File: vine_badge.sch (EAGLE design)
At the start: 44 parts

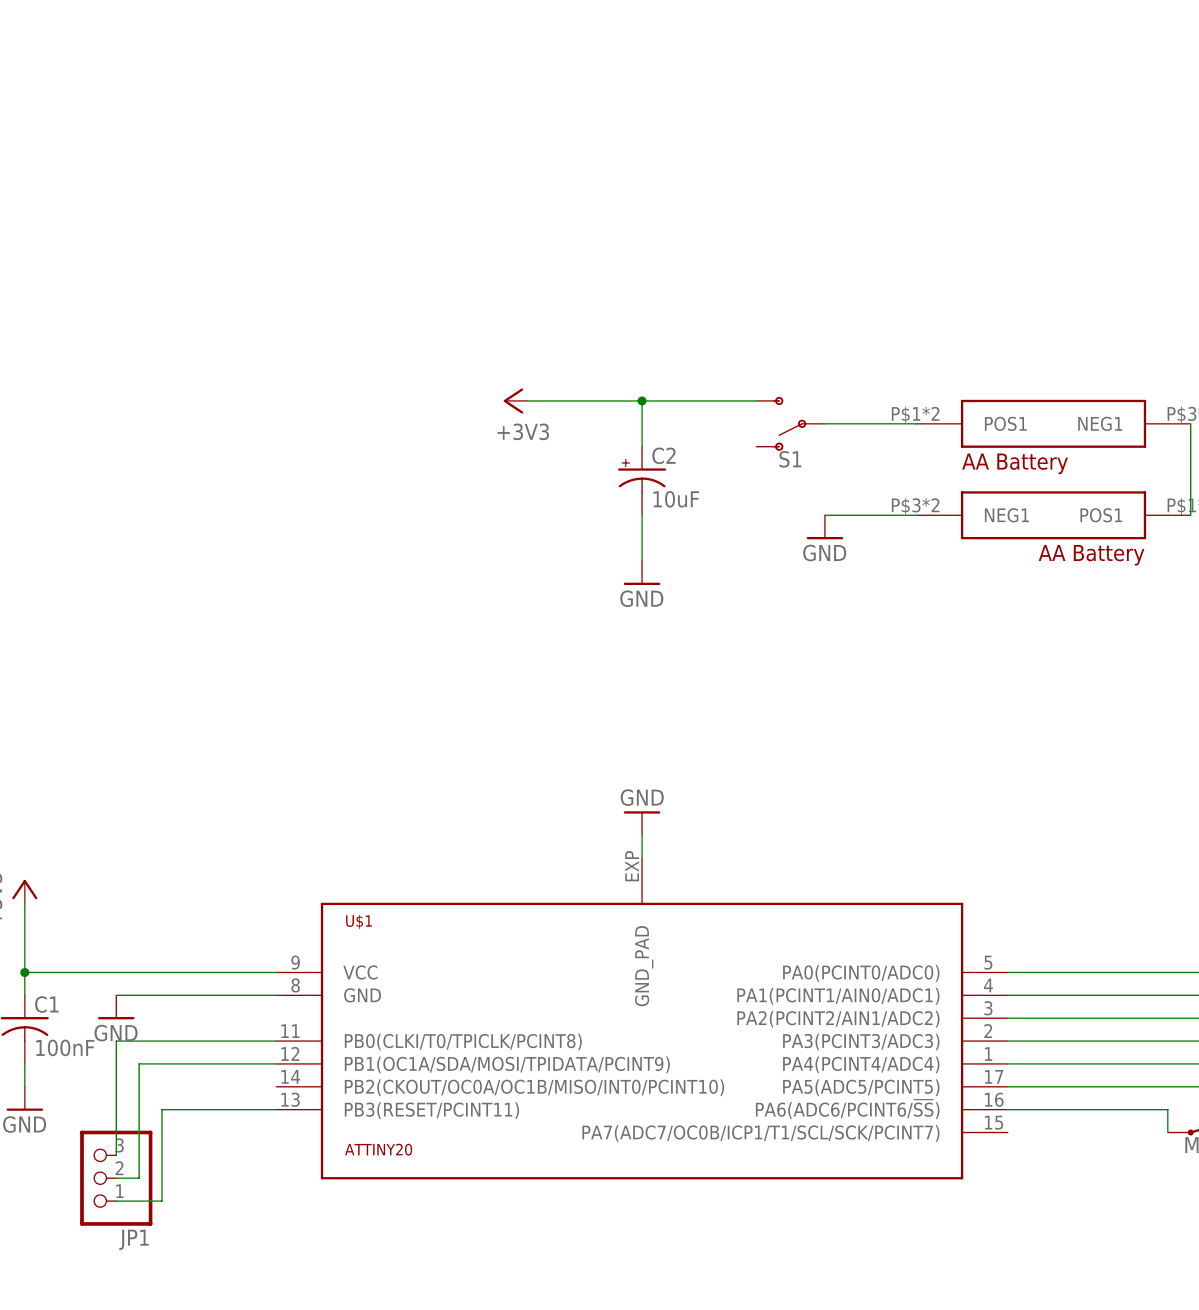
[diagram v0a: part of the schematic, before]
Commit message: final checking phase
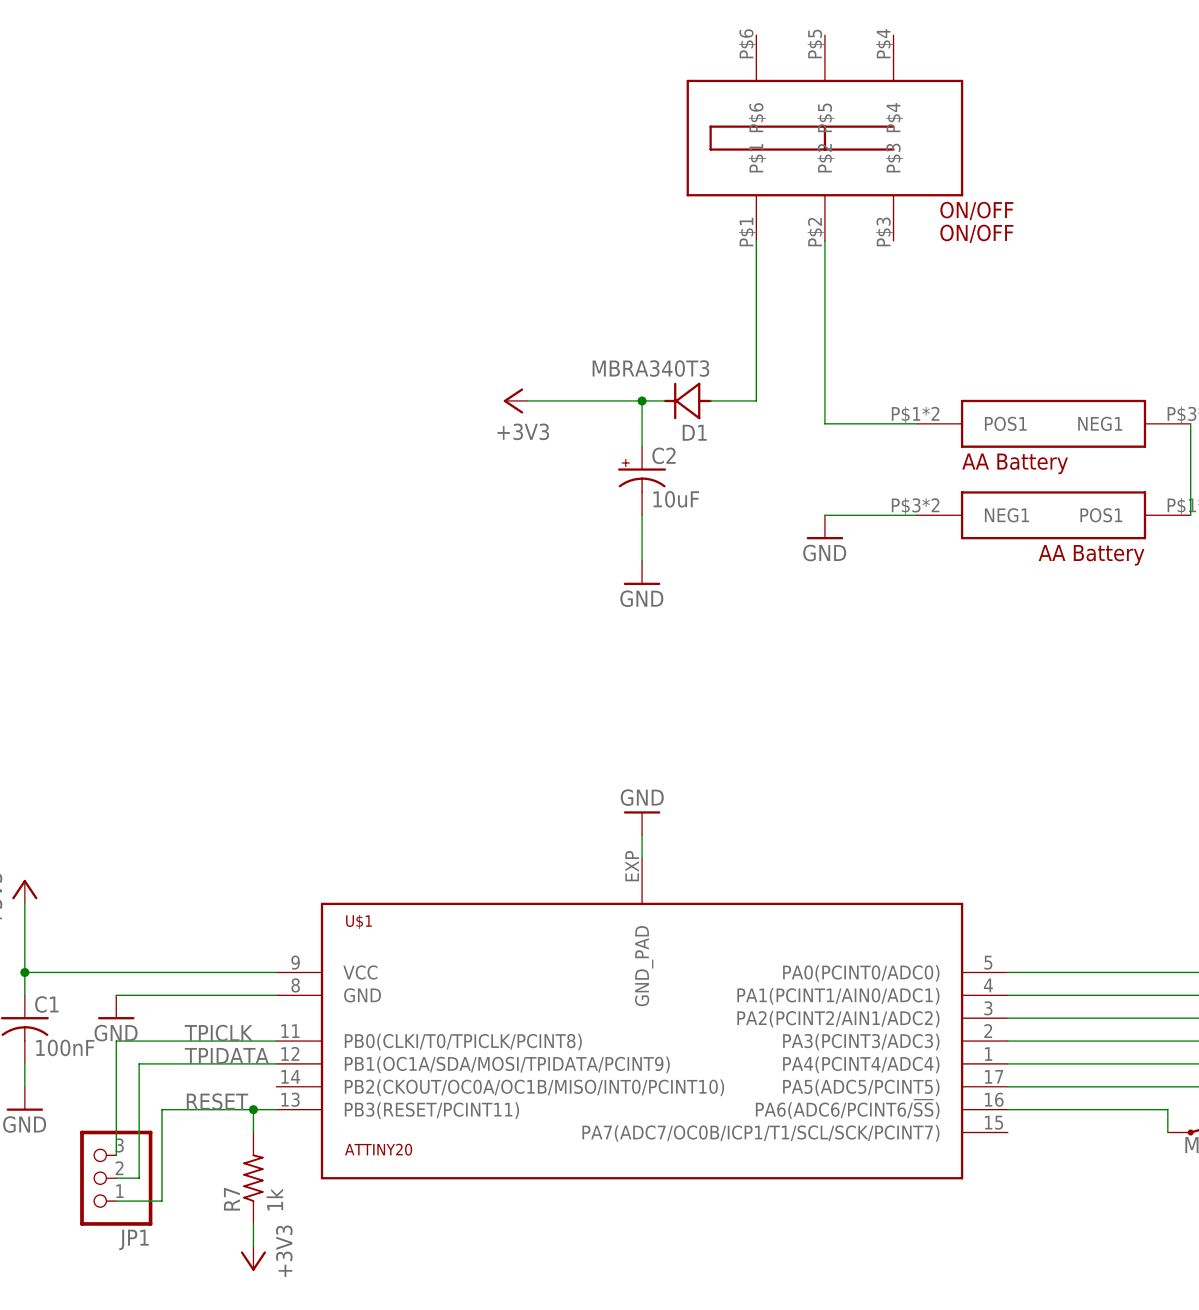
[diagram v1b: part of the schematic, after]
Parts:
- removed S1: (no value), SparkFun-Switches:SWITCH-SPDT-SMD-AYZ0202
- added D1: MBRA340T3, diode:MBRA340T3
- added ON/OFF: ON/OFF, VineBadge:SMT_DPDT
- added R7: 1k, resistor:R-US_R0603
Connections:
- net N$10 renamed TPIDATA
- net N$8 renamed TPICLK
- removed net N$12: JP1.1, U$1G$2.PB3(RESET/PCINT11)
- new net N$20: D1.A, ON/OFF.P$1
- new net RESET: JP1.1, R7.2, U$1G$2.PB3(RESET/PCINT11)
- net +3V3: now also D1.C, R7.1; no longer S1.S
- net N$19: now also ON/OFF.P$2; no longer S1.P
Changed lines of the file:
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@@
 <part name="C1" library="resistor" library_urn="urn:adsk.eagle:library:348" deviceset="C-US" device="C0603" package3d_urn="urn:adsk.eagle:package:23616/2" value="100nF"/>
 <part name="GND3" library="supply1" library_urn="urn:adsk.eagle:library:371" deviceset="GND" device=""/>
-<part name="S1" library="SparkFun-Switches" library_urn="urn:adsk.eagle:library:535" deviceset="SWITCH-SPDT" device="-SMD-AYZ0202" package3d_urn="urn:adsk.eagle:package:40160/1"/>
 <part name="+3V2" library="supply1" library_urn="urn:adsk.eagle:library:371" deviceset="+3V3" device=""/>
 <part name="GND4" library="supply1" library_urn="urn:adsk.eagle:library:371" deviceset="GND" device=""/>
@@
 <part name="S2" library="SparkFun-Switches" library_urn="urn:adsk.eagle:library:535" deviceset="MOMENTARY-SWITCH-SPST" device="-SMD-6.0X3.5MM" package3d_urn="urn:adsk.eagle:package:40165/1" value="MODE"/>
 <part name="JP1" library="pinhead" library_urn="urn:adsk.eagle:library:325" deviceset="PINHD-1X3" device="" package3d_urn="urn:adsk.eagle:package:22458/2"/>
+<part name="D1" library="diode" library_urn="urn:adsk.eagle:library:210" deviceset="MBRA340T3" device="" package3d_urn="urn:adsk.eagle:package:43460/3"/>
+<part name="R7" library="resistor" library_urn="urn:adsk.eagle:library:348" deviceset="R-US_" device="R0603" package3d_urn="urn:adsk.eagle:package:23555/2" value="1k"/>
+<part name="+3V3" library="supply1" library_urn="urn:adsk.eagle:library:371" deviceset="+3V3" device=""/>
+<part name="ON/OFF" library="VineBadge" deviceset="SMT_DPDT" device="" value="ON/OFF"/>
 </parts>
 <sheets>
@@
 <attribute name="VALUE" x="17.78" y="25.4" size="1.778" layer="96"/>
 </instance>
-<instance part="S1" gate="1" x="106.68" y="104.14" smashed="yes" rot="R180">
-<attribute name="NAME" x="105.41" y="101.092" size="1.778" layer="95" font="vector" rot="R180" align="bottom-center"/>
-<attribute name="VALUE" x="105.664" y="107.442" size="1.778" layer="96" font="vector" rot="R180" align="top-center"/>
-</instance>
 <instance part="+3V2" gate="G$1" x="73.66" y="106.68" smashed="yes" rot="R90">
 <attribute name="VALUE" x="78.74" y="104.14" size="1.778" layer="96" rot="R180"/>
@@
 <attribute name="NAME" x="34.29" y="14.605" size="1.778" layer="95" rot="R180"/>
 <attribute name="VALUE" x="34.29" y="27.94" size="1.778" layer="96" rot="R180"/>
+</instance>
+<instance part="D1" gate="G$1" x="93.98" y="106.68" smashed="yes" rot="R180">
+<attribute name="NAME" x="96.2914" y="104.0384" size="1.778" layer="95" rot="R180"/>
+<attribute name="VALUE" x="96.5454" y="111.1758" size="1.778" layer="96" rot="R180"/>
+</instance>
+<instance part="R7" gate="G$1" x="45.72" y="20.32" smashed="yes" rot="R90">
+<attribute name="NAME" x="44.2214" y="16.51" size="1.778" layer="95" rot="R90"/>
+<attribute name="VALUE" x="49.022" y="16.51" size="1.778" layer="96" rot="R90"/>
+</instance>
+<instance part="+3V3" gate="G$1" x="45.72" y="10.16" smashed="yes" rot="R180">
+<attribute name="VALUE" x="48.26" y="15.24" size="1.778" layer="96" rot="R270"/>
+</instance>
+<instance part="ON/OFF" gate="G$1" x="109.22" y="129.54" smashed="yes">
+<attribute name="NAME" x="121.92" y="127" size="1.778" layer="94"/>
+<attribute name="VALUE" x="121.92" y="124.46" size="1.778" layer="94"/>
 </instance>
 </instances>
@@
 </segment>
 <segment>
-<pinref part="S1" gate="1" pin="S"/>
 <pinref part="+3V2" gate="G$1" pin="+3V3"/>
-<wire x1="101.6" y1="106.68" x2="88.9" y2="106.68" width="0.1524" layer="91"/>
 <pinref part="C2" gate="G$1" pin="+"/>
 <wire x1="88.9" y1="106.68" x2="76.2" y2="106.68" width="0.1524" layer="91"/>
 <wire x1="88.9" y1="101.6" x2="88.9" y2="106.68" width="0.1524" layer="91"/>
+<pinref part="D1" gate="G$1" pin="C"/>
+<wire x1="91.44" y1="106.68" x2="88.9" y2="106.68" width="0.1524" layer="91"/>
 <junction x="88.9" y="106.68"/>
+</segment>
+<segment>
+<pinref part="R7" gate="G$1" pin="1"/>
+<pinref part="+3V3" gate="G$1" pin="+3V3"/>
+<wire x1="45.72" y1="15.24" x2="45.72" y2="12.7" width="0.1524" layer="91"/>
 </segment>
 </net>
@@
 </segment>
 </net>
-<net name="N$8" class="0">
+<net name="TPICLK" class="0">
 <segment>
 <pinref part="U$1" gate="G$2" pin="PB0(CLKI/T0/TPICLK/PCINT8)"/>
@@
 <pinref part="JP1" gate="A" pin="3"/>
 <wire x1="30.48" y1="35.56" x2="30.48" y2="22.86" width="0.1524" layer="91"/>
-</segment>
-</net>
-<net name="N$10" class="0">
+<label x="38.1" y="35.56" size="1.778" layer="95"/>
+</segment>
+</net>
+<net name="TPIDATA" class="0">
 <segment>
 <pinref part="U$1" gate="G$2" pin="PB1(OC1A/SDA/MOSI/TPIDATA/PCINT9)"/>
@@
 <pinref part="JP1" gate="A" pin="2"/>
 <wire x1="33.02" y1="20.32" x2="30.48" y2="20.32" width="0.1524" layer="91"/>
-</segment>
-</net>
-<net name="N$12" class="0">
+<label x="38.1" y="33.02" size="1.778" layer="95"/>
+</segment>
+</net>
+<net name="RESET" class="0">
 <segment>
 <pinref part="U$1" gate="G$2" pin="PB3(RESET/PCINT11)"/>
-<wire x1="48.26" y1="27.94" x2="35.56" y2="27.94" width="0.1524" layer="91"/>
+<wire x1="48.26" y1="27.94" x2="45.72" y2="27.94" width="0.1524" layer="91"/>
 <pinref part="JP1" gate="A" pin="1"/>
+<wire x1="45.72" y1="27.94" x2="35.56" y2="27.94" width="0.1524" layer="91"/>
 <wire x1="35.56" y1="27.94" x2="35.56" y2="17.78" width="0.1524" layer="91"/>
 <wire x1="35.56" y1="17.78" x2="30.48" y2="17.78" width="0.1524" layer="91"/>
+<label x="38.1" y="27.94" size="1.778" layer="95"/>
+<pinref part="R7" gate="G$1" pin="2"/>
+<wire x1="45.72" y1="25.4" x2="45.72" y2="27.94" width="0.1524" layer="91"/>
+<junction x="45.72" y="27.94"/>
 </segment>
 </net>
@@
 <pinref part="U$2" gate="G$1" pin="POS1"/>
 <wire x1="119.38" y1="104.14" x2="109.22" y2="104.14" width="0.1524" layer="91"/>
-<pinref part="S1" gate="1" pin="P"/>
+<pinref part="ON/OFF" gate="G$1" pin="P$2"/>
+<wire x1="109.22" y1="104.14" x2="109.22" y2="124.46" width="0.1524" layer="91"/>
 </segment>
 </net>
@@
 </segment>
 </net>
+<net name="N$20" class="0">
+<segment>
+<pinref part="D1" gate="G$1" pin="A"/>
+<wire x1="96.52" y1="106.68" x2="101.6" y2="106.68" width="0.1524" layer="91"/>
+<pinref part="ON/OFF" gate="G$1" pin="P$1"/>
+<wire x1="101.6" y1="124.46" x2="101.6" y2="106.68" width="0.1524" layer="91"/>
+</segment>
+</net>
